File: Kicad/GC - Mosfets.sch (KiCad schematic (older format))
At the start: 15 parts, among them Q1 IRFB7530, Q2 IRFB7530, Q3 IRFB7530, Q4 IRFB7530, Q5 IRFB7530, Q6 IRFB7530

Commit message: Passives changed from 0805 to 0603
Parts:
- Q1, Q2, Q3, Q4, Q5, Q6: footprint TO_SOT_Packages_THT:TO-220-3_Horizontal -> Romain:TO-220-3_Horizontal
- R1, R10, R11, R12, R13, R2, R7, R8, R9: footprint Resistors_SMD:R_0805 -> Resistors_SMD:R_0603
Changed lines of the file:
@@
 F 0 "R13" V 7350 4150 50  0000 C CNN
 F 1 "39k" V 7250 4150 50  0000 C CNN
-F 2 "Resistors_SMD:R_0805" H 7250 4150 60  0001 C CNN
+F 2 "Resistors_SMD:R_0603" H 7250 4150 60  0001 C CNN
 F 3 "" H 7250 4150 60  0001 C CNN
 	1    7250 4150
@@
 F 0 "R7" V 4200 4150 50  0000 C CNN
 F 1 "39k" V 4100 4150 50  0000 C CNN
-F 2 "Resistors_SMD:R_0805" H 4100 4150 60  0001 C CNN
+F 2 "Resistors_SMD:R_0603" H 4100 4150 60  0001 C CNN
 F 3 "" H 4100 4150 60  0001 C CNN
 	1    4100 4150
@@
 F 0 "Q1" H 4210 3070 60  0000 R CNN
 F 1 "IRFB7530" V 4450 3100 60  0000 R CNN
-F 2 "TO_SOT_Packages_THT:TO-220-3_Horizontal" H 4200 2900 60  0001 C CNN
+F 2 "Romain:TO-220-3_Horizontal" H 4200 2900 60  0001 C CNN
 F 3 "IRFB7530" H 4200 2900 60  0001 C CNN
 F 4 "IRFB7530" H 4200 2900 50  0001 C CNN "mfg#"
@@
 F 0 "Q2" H 4210 4020 60  0000 R CNN
 F 1 "IRFB7530" V 4450 4050 60  0000 R CNN
-F 2 "TO_SOT_Packages_THT:TO-220-3_Horizontal" H 4200 3850 60  0001 C CNN
+F 2 "Romain:TO-220-3_Horizontal" H 4200 3850 60  0001 C CNN
 F 3 "IRFB7530" H 4200 3850 60  0001 C CNN
 F 4 "IRFB7530" H 4200 3850 50  0001 C CNN "mfg#"
@@
 F 0 "R2" V 3750 3850 50  0000 C CNN
 F 1 "4R7" V 3650 3850 50  0000 C CNN
-F 2 "Resistors_SMD:R_0805" H 3650 3850 60  0001 C CNN
+F 2 "Resistors_SMD:R_0603" H 3650 3850 60  0001 C CNN
 F 3 "" H 3650 3850 60  0001 C CNN
 	1    3650 3850
@@
 F 0 "R1" V 3750 2900 50  0000 C CNN
 F 1 "4R7" V 3650 2900 50  0000 C CNN
-F 2 "Resistors_SMD:R_0805" H 3650 2900 60  0001 C CNN
+F 2 "Resistors_SMD:R_0603" H 3650 2900 60  0001 C CNN
 F 3 "" H 3650 2900 60  0001 C CNN
 	1    3650 2900
@@
 F 0 "R8" V 5300 2900 50  0000 C CNN
 F 1 "4R7" V 5200 2900 50  0000 C CNN
-F 2 "Resistors_SMD:R_0805" H 5200 2900 60  0001 C CNN
+F 2 "Resistors_SMD:R_0603" H 5200 2900 60  0001 C CNN
 F 3 "" H 5200 2900 60  0001 C CNN
 	1    5200 2900
@@
 F 0 "R9" V 5300 3850 50  0000 C CNN
 F 1 "4R7" V 5200 3850 50  0000 C CNN
-F 2 "Resistors_SMD:R_0805" H 5200 3850 60  0001 C CNN
+F 2 "Resistors_SMD:R_0603" H 5200 3850 60  0001 C CNN
 F 3 "" H 5200 3850 60  0001 C CNN
 	1    5200 3850
@@
 F 0 "Q4" H 5760 4020 60  0000 R CNN
 F 1 "IRFB7530" V 6000 4050 60  0000 R CNN
-F 2 "TO_SOT_Packages_THT:TO-220-3_Horizontal" H 5750 3850 60  0001 C CNN
+F 2 "Romain:TO-220-3_Horizontal" H 5750 3850 60  0001 C CNN
 F 3 "IRFB7530" H 5750 3850 60  0001 C CNN
 F 4 "IRFB7530" H 5750 3850 50  0001 C CNN "mfg#"
@@
 F 0 "Q3" H 5760 3070 60  0000 R CNN
 F 1 "IRFB7530" V 6000 3100 60  0000 R CNN
-F 2 "TO_SOT_Packages_THT:TO-220-3_Horizontal" H 5750 2900 60  0001 C CNN
+F 2 "Romain:TO-220-3_Horizontal" H 5750 2900 60  0001 C CNN
 F 3 "IRFB7530" H 5750 2900 60  0001 C CNN
 F 4 "IRFB7530" H 5750 2900 50  0001 C CNN "mfg#"
@@
 F 0 "Q5" H 7360 3070 60  0000 R CNN
 F 1 "IRFB7530" V 7600 3100 60  0000 R CNN
-F 2 "TO_SOT_Packages_THT:TO-220-3_Horizontal" H 7350 2900 60  0001 C CNN
+F 2 "Romain:TO-220-3_Horizontal" H 7350 2900 60  0001 C CNN
 F 3 "IRFB7530" H 7350 2900 60  0001 C CNN
 F 4 "IRFB7530" H 7350 2900 50  0001 C CNN "mfg#"
@@
 F 0 "Q6" H 7360 4020 60  0000 R CNN
 F 1 "IRFB7530" V 7600 4050 60  0000 R CNN
-F 2 "TO_SOT_Packages_THT:TO-220-3_Horizontal" H 7350 3850 60  0001 C CNN
+F 2 "Romain:TO-220-3_Horizontal" H 7350 3850 60  0001 C CNN
 F 3 "IRFB7530" H 7350 3850 60  0001 C CNN
 F 4 "IRFB7530" H 7350 3850 50  0001 C CNN "mfg#"
@@
 F 0 "R12" V 6900 3850 50  0000 C CNN
 F 1 "4R7" V 6800 3850 50  0000 C CNN
-F 2 "Resistors_SMD:R_0805" H 6800 3850 60  0001 C CNN
+F 2 "Resistors_SMD:R_0603" H 6800 3850 60  0001 C CNN
 F 3 "" H 6800 3850 60  0001 C CNN
 	1    6800 3850
@@
 F 0 "R11" V 6900 2900 50  0000 C CNN
 F 1 "4R7" V 6800 2900 50  0000 C CNN
-F 2 "Resistors_SMD:R_0805" H 6800 2900 60  0001 C CNN
+F 2 "Resistors_SMD:R_0603" H 6800 2900 60  0001 C CNN
 F 3 "" H 6800 2900 60  0001 C CNN
 	1    6800 2900
@@
 F 0 "R10" V 5100 4150 50  0000 C CNN
 F 1 "39k" V 5200 4150 50  0000 C CNN
-F 2 "Resistors_SMD:R_0805" H 5200 4150 60  0001 C CNN
+F 2 "Resistors_SMD:R_0603" H 5200 4150 60  0001 C CNN
 F 3 "" H 5200 4150 60  0001 C CNN
 	1    5200 4150

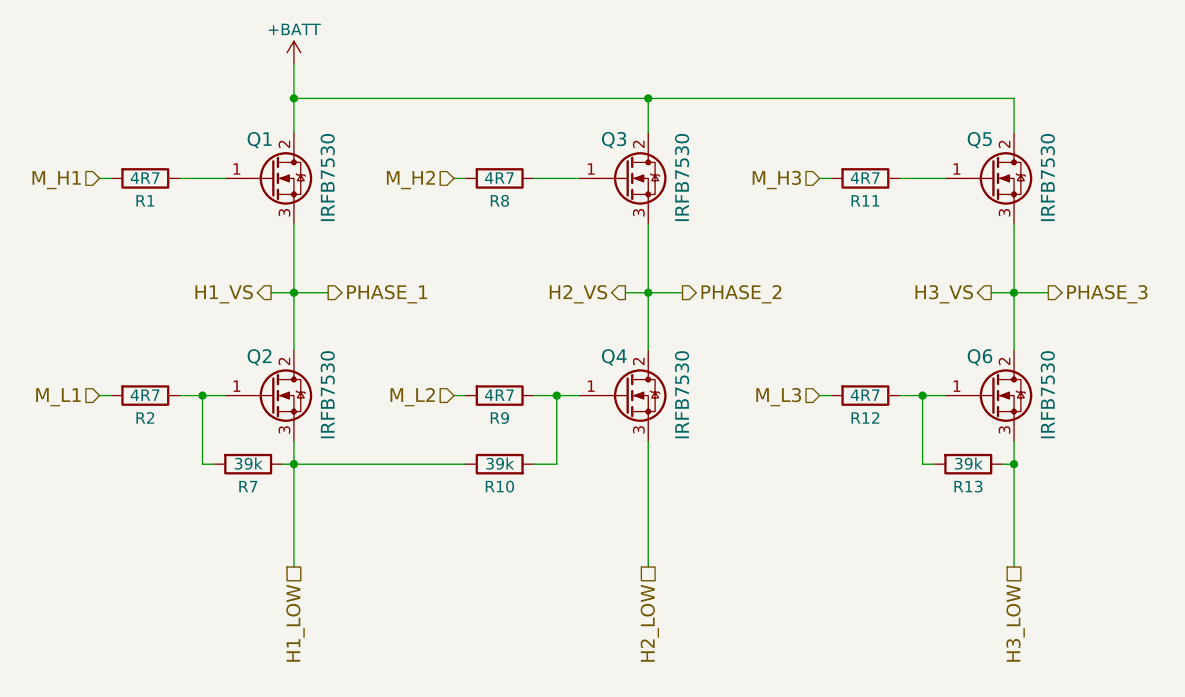
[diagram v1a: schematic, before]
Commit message: Components placed
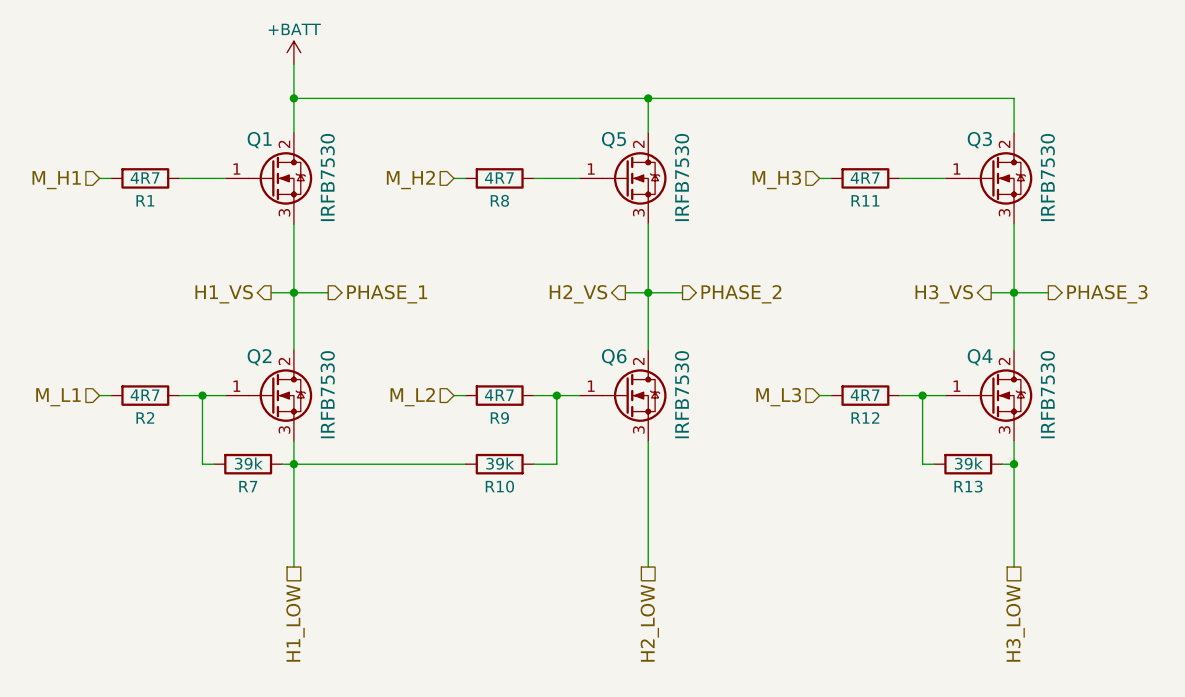
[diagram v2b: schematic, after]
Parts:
- renumbered Q5 to Q3, Q6 to Q4, Q3 to Q5, Q4 to Q6
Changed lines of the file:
@@
 $EndComp
 $Comp
-L Device:Q_NMOS_GDS Q4
+L Device:Q_NMOS_GDS Q6
 U 1 1 53F8E66C
 P 5750 3850
-F 0 "Q4" H 5760 4020 60  0000 R CNN
+F 0 "Q6" H 5760 4020 60  0000 R CNN
 F 1 "IRFB7530" V 6000 4050 60  0000 R CNN
 F 2 "Romain:TO-220-3_Horizontal" H 5750 3850 60  0001 C CNN
@@
 $EndComp
 $Comp
-L Device:Q_NMOS_GDS Q3
+L Device:Q_NMOS_GDS Q5
 U 1 1 53F8E673
 P 5750 2900
-F 0 "Q3" H 5760 3070 60  0000 R CNN
+F 0 "Q5" H 5760 3070 60  0000 R CNN
 F 1 "IRFB7530" V 6000 3100 60  0000 R CNN
 F 2 "Romain:TO-220-3_Horizontal" H 5750 2900 60  0001 C CNN
@@
 $EndComp
 $Comp
-L Device:Q_NMOS_GDS Q5
+L Device:Q_NMOS_GDS Q3
 U 1 1 53F8E67A
 P 7350 2900
-F 0 "Q5" H 7360 3070 60  0000 R CNN
+F 0 "Q3" H 7360 3070 60  0000 R CNN
 F 1 "IRFB7530" V 7600 3100 60  0000 R CNN
 F 2 "Romain:TO-220-3_Horizontal" H 7350 2900 60  0001 C CNN
@@
 $EndComp
 $Comp
-L Device:Q_NMOS_GDS Q6
+L Device:Q_NMOS_GDS Q4
 U 1 1 53F8E681
 P 7350 3850
-F 0 "Q6" H 7360 4020 60  0000 R CNN
+F 0 "Q4" H 7360 4020 60  0000 R CNN
 F 1 "IRFB7530" V 7600 4050 60  0000 R CNN
 F 2 "Romain:TO-220-3_Horizontal" H 7350 3850 60  0001 C CNN

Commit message: Adjusting capacitor size/value
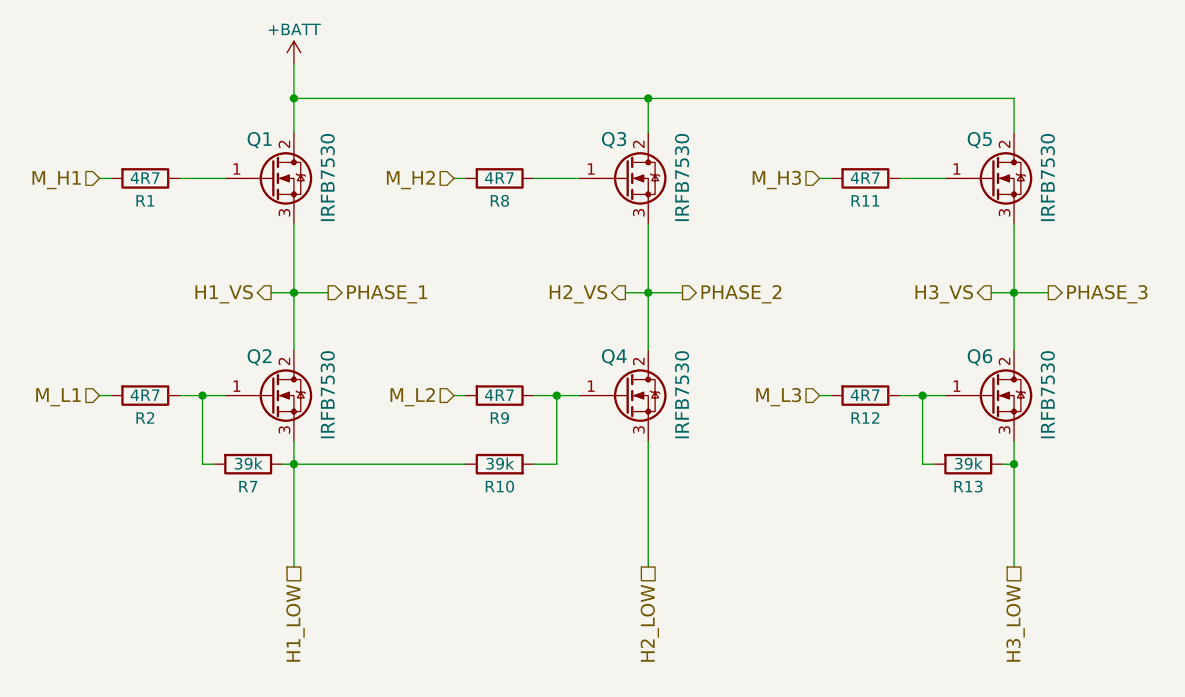
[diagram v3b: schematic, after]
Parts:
- renumbered Q5 to Q3, Q6 to Q4, Q3 to Q5, Q4 to Q6
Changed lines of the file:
@@
 $EndComp
 $Comp
-L Device:Q_NMOS_GDS Q6
+L Device:Q_NMOS_GDS Q4
 U 1 1 53F8E66C
 P 5750 3850
-F 0 "Q6" H 5760 4020 60  0000 R CNN
+F 0 "Q4" H 5760 4020 60  0000 R CNN
 F 1 "IRFB7530" V 6000 4050 60  0000 R CNN
 F 2 "Romain:TO-220-3_Horizontal" H 5750 3850 60  0001 C CNN
@@
 $EndComp
 $Comp
-L Device:Q_NMOS_GDS Q5
+L Device:Q_NMOS_GDS Q3
 U 1 1 53F8E673
 P 5750 2900
-F 0 "Q5" H 5760 3070 60  0000 R CNN
+F 0 "Q3" H 5760 3070 60  0000 R CNN
 F 1 "IRFB7530" V 6000 3100 60  0000 R CNN
 F 2 "Romain:TO-220-3_Horizontal" H 5750 2900 60  0001 C CNN
@@
 $EndComp
 $Comp
-L Device:Q_NMOS_GDS Q3
+L Device:Q_NMOS_GDS Q5
 U 1 1 53F8E67A
 P 7350 2900
-F 0 "Q3" H 7360 3070 60  0000 R CNN
+F 0 "Q5" H 7360 3070 60  0000 R CNN
 F 1 "IRFB7530" V 7600 3100 60  0000 R CNN
 F 2 "Romain:TO-220-3_Horizontal" H 7350 2900 60  0001 C CNN
@@
 $EndComp
 $Comp
-L Device:Q_NMOS_GDS Q4
+L Device:Q_NMOS_GDS Q6
 U 1 1 53F8E681
 P 7350 3850
-F 0 "Q4" H 7360 4020 60  0000 R CNN
+F 0 "Q6" H 7360 4020 60  0000 R CNN
 F 1 "IRFB7530" V 7600 4050 60  0000 R CNN
 F 2 "Romain:TO-220-3_Horizontal" H 7350 3850 60  0001 C CNN

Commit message: Fixed libraries issues
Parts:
- Q1, Q2, Q3, Q4, Q5, Q6: footprint Romain:TO-220-3_Horizontal -> Gouach-Controller:TO-220-3_Horizontal; symbol Device:Q_NMOS_GDS -> Gouach_Controller-rescue:Q_NMOS_GDS-Device
- R1, R10, R11, R12, R13, R2, R7, R8, R9: footprint Resistors_SMD:R_0603 -> Resistor_SMD:R_0603_1608Metric; symbol Device:R -> Gouach_Controller-rescue:R-Device
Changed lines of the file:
@@
 $EndDescr
 $Comp
-L Device:R R13
+L Gouach_Controller-rescue:R-Device R13
 U 1 1 53F8E60B
 P 7250 4150
 F 0 "R13" V 7350 4150 50  0000 C CNN
 F 1 "39k" V 7250 4150 50  0000 C CNN
-F 2 "Resistors_SMD:R_0603" H 7250 4150 60  0001 C CNN
+F 2 "Resistor_SMD:R_0603_1608Metric" H 7250 4150 60  0001 C CNN
 F 3 "" H 7250 4150 60  0001 C CNN
 	1    7250 4150
@@
 $EndComp
 $Comp
-L Device:R R7
+L Gouach_Controller-rescue:R-Device R7
 U 1 1 53F8E612
 P 4100 4150
 F 0 "R7" V 4200 4150 50  0000 C CNN
 F 1 "39k" V 4100 4150 50  0000 C CNN
-F 2 "Resistors_SMD:R_0603" H 4100 4150 60  0001 C CNN
+F 2 "Resistor_SMD:R_0603_1608Metric" H 4100 4150 60  0001 C CNN
 F 3 "" H 4100 4150 60  0001 C CNN
 	1    4100 4150
@@
 $EndComp
 $Comp
-L Device:Q_NMOS_GDS Q1
+L Gouach_Controller-rescue:Q_NMOS_GDS-Device Q1
 U 1 1 53F8E63D
 P 4200 2900
 F 0 "Q1" H 4210 3070 60  0000 R CNN
 F 1 "IRFB7530" V 4450 3100 60  0000 R CNN
-F 2 "Romain:TO-220-3_Horizontal" H 4200 2900 60  0001 C CNN
+F 2 "Gouach-Controller:TO-220-3_Horizontal" H 4200 2900 60  0001 C CNN
 F 3 "IRFB7530" H 4200 2900 60  0001 C CNN
 F 4 "IRFB7530" H 4200 2900 50  0001 C CNN "mfg#"
@@
 $EndComp
 $Comp
-L Device:Q_NMOS_GDS Q2
+L Gouach_Controller-rescue:Q_NMOS_GDS-Device Q2
 U 1 1 53F8E644
 P 4200 3850
 F 0 "Q2" H 4210 4020 60  0000 R CNN
 F 1 "IRFB7530" V 4450 4050 60  0000 R CNN
-F 2 "Romain:TO-220-3_Horizontal" H 4200 3850 60  0001 C CNN
+F 2 "Gouach-Controller:TO-220-3_Horizontal" H 4200 3850 60  0001 C CNN
 F 3 "IRFB7530" H 4200 3850 60  0001 C CNN
 F 4 "IRFB7530" H 4200 3850 50  0001 C CNN "mfg#"
@@
 $EndComp
 $Comp
-L Device:R R2
+L Gouach_Controller-rescue:R-Device R2
 U 1 1 53F8E64B
 P 3650 3850
 F 0 "R2" V 3750 3850 50  0000 C CNN
 F 1 "4R7" V 3650 3850 50  0000 C CNN
-F 2 "Resistors_SMD:R_0603" H 3650 3850 60  0001 C CNN
+F 2 "Resistor_SMD:R_0603_1608Metric" H 3650 3850 60  0001 C CNN
 F 3 "" H 3650 3850 60  0001 C CNN
 	1    3650 3850
@@
 $EndComp
 $Comp
-L Device:R R1
+L Gouach_Controller-rescue:R-Device R1
 U 1 1 53F8E652
 P 3650 2900
 F 0 "R1" V 3750 2900 50  0000 C CNN
 F 1 "4R7" V 3650 2900 50  0000 C CNN
-F 2 "Resistors_SMD:R_0603" H 3650 2900 60  0001 C CNN
+F 2 "Resistor_SMD:R_0603_1608Metric" H 3650 2900 60  0001 C CNN
 F 3 "" H 3650 2900 60  0001 C CNN
 	1    3650 2900
@@
 $EndComp
 $Comp
-L Device:R R8
+L Gouach_Controller-rescue:R-Device R8
 U 1 1 53F8E65E
 P 5200 2900
 F 0 "R8" V 5300 2900 50  0000 C CNN
 F 1 "4R7" V 5200 2900 50  0000 C CNN
-F 2 "Resistors_SMD:R_0603" H 5200 2900 60  0001 C CNN
+F 2 "Resistor_SMD:R_0603_1608Metric" H 5200 2900 60  0001 C CNN
 F 3 "" H 5200 2900 60  0001 C CNN
 	1    5200 2900
@@
 $EndComp
 $Comp
-L Device:R R9
+L Gouach_Controller-rescue:R-Device R9
 U 1 1 53F8E665
 P 5200 3850
 F 0 "R9" V 5300 3850 50  0000 C CNN
 F 1 "4R7" V 5200 3850 50  0000 C CNN
-F 2 "Resistors_SMD:R_0603" H 5200 3850 60  0001 C CNN
+F 2 "Resistor_SMD:R_0603_1608Metric" H 5200 3850 60  0001 C CNN
 F 3 "" H 5200 3850 60  0001 C CNN
 	1    5200 3850
@@
 $EndComp
 $Comp
-L Device:Q_NMOS_GDS Q4
+L Gouach_Controller-rescue:Q_NMOS_GDS-Device Q4
 U 1 1 53F8E66C
 P 5750 3850
 F 0 "Q4" H 5760 4020 60  0000 R CNN
 F 1 "IRFB7530" V 6000 4050 60  0000 R CNN
-F 2 "Romain:TO-220-3_Horizontal" H 5750 3850 60  0001 C CNN
+F 2 "Gouach-Controller:TO-220-3_Horizontal" H 5750 3850 60  0001 C CNN
 F 3 "IRFB7530" H 5750 3850 60  0001 C CNN
 F 4 "IRFB7530" H 5750 3850 50  0001 C CNN "mfg#"
@@
 $EndComp
 $Comp
-L Device:Q_NMOS_GDS Q3
+L Gouach_Controller-rescue:Q_NMOS_GDS-Device Q3
 U 1 1 53F8E673
 P 5750 2900
 F 0 "Q3" H 5760 3070 60  0000 R CNN
 F 1 "IRFB7530" V 6000 3100 60  0000 R CNN
-F 2 "Romain:TO-220-3_Horizontal" H 5750 2900 60  0001 C CNN
+F 2 "Gouach-Controller:TO-220-3_Horizontal" H 5750 2900 60  0001 C CNN
 F 3 "IRFB7530" H 5750 2900 60  0001 C CNN
 F 4 "IRFB7530" H 5750 2900 50  0001 C CNN "mfg#"
@@
 $EndComp
 $Comp
-L Device:Q_NMOS_GDS Q5
+L Gouach_Controller-rescue:Q_NMOS_GDS-Device Q5
 U 1 1 53F8E67A
 P 7350 2900
 F 0 "Q5" H 7360 3070 60  0000 R CNN
 F 1 "IRFB7530" V 7600 3100 60  0000 R CNN
-F 2 "Romain:TO-220-3_Horizontal" H 7350 2900 60  0001 C CNN
+F 2 "Gouach-Controller:TO-220-3_Horizontal" H 7350 2900 60  0001 C CNN
 F 3 "IRFB7530" H 7350 2900 60  0001 C CNN
 F 4 "IRFB7530" H 7350 2900 50  0001 C CNN "mfg#"
@@
 $EndComp
 $Comp
-L Device:Q_NMOS_GDS Q6
+L Gouach_Controller-rescue:Q_NMOS_GDS-Device Q6
 U 1 1 53F8E681
 P 7350 3850
 F 0 "Q6" H 7360 4020 60  0000 R CNN
 F 1 "IRFB7530" V 7600 4050 60  0000 R CNN
-F 2 "Romain:TO-220-3_Horizontal" H 7350 3850 60  0001 C CNN
+F 2 "Gouach-Controller:TO-220-3_Horizontal" H 7350 3850 60  0001 C CNN
 F 3 "IRFB7530" H 7350 3850 60  0001 C CNN
 F 4 "IRFB7530" H 7350 3850 50  0001 C CNN "mfg#"
@@
 $EndComp
 $Comp
-L Device:R R12
+L Gouach_Controller-rescue:R-Device R12
 U 1 1 53F8E688
 P 6800 3850
 F 0 "R12" V 6900 3850 50  0000 C CNN
 F 1 "4R7" V 6800 3850 50  0000 C CNN
-F 2 "Resistors_SMD:R_0603" H 6800 3850 60  0001 C CNN
+F 2 "Resistor_SMD:R_0603_1608Metric" H 6800 3850 60  0001 C CNN
 F 3 "" H 6800 3850 60  0001 C CNN
 	1    6800 3850
@@
 $EndComp
 $Comp
-L Device:R R11
+L Gouach_Controller-rescue:R-Device R11
 U 1 1 53F8E68F
 P 6800 2900
 F 0 "R11" V 6900 2900 50  0000 C CNN
 F 1 "4R7" V 6800 2900 50  0000 C CNN
-F 2 "Resistors_SMD:R_0603" H 6800 2900 60  0001 C CNN
+F 2 "Resistor_SMD:R_0603_1608Metric" H 6800 2900 60  0001 C CNN
 F 3 "" H 6800 2900 60  0001 C CNN
 	1    6800 2900
@@
 $EndComp
 $Comp
-L Device:R R10
+L Gouach_Controller-rescue:R-Device R10
 U 1 1 53F8E69C
 P 5200 4150
 F 0 "R10" V 5100 4150 50  0000 C CNN
 F 1 "39k" V 5200 4150 50  0000 C CNN
-F 2 "Resistors_SMD:R_0603" H 5200 4150 60  0001 C CNN
+F 2 "Resistor_SMD:R_0603_1608Metric" H 5200 4150 60  0001 C CNN
 F 3 "" H 5200 4150 60  0001 C CNN
 	1    5200 4150
@@
 	7050 4150 7100 4150
 $Comp
-L power:+BATT #PWR0126
+L Gouach_Controller-rescue:+BATT-power #PWR0126
 U 1 1 5F21FCD0
 P 4300 2400

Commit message: Add Mouser order number
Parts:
- Q1, Q2, Q3, Q4, Q5, Q6: Mouser (none) -> 942-IRFB7530PBF; mfg# IRFB7530 -> (none)
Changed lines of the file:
@@
 F 1 "IRFB7530" V 4450 3100 60  0000 R CNN
 F 2 "Gouach-Controller:TO-220-3_Horizontal" H 4200 2900 60  0001 C CNN
-F 3 "IRFB7530" H 4200 2900 60  0001 C CNN
-F 4 "IRFB7530" H 4200 2900 50  0001 C CNN "mfg#"
+F 3 "https://www.infineon.com/dgdl/irfs7530pbf.pdf?fileId=5546d462533600a4015364c3d98429c3" H 4200 2900 60  0001 C CNN
+F 4 "" H 4200 2900 50  0001 C CNN "mfg#"
+F 5 "942-IRFB7530PBF " H 4200 2900 50  0001 C CNN "Mouser"
 	1    4200 2900
 	1    0    0    -1
@@
 F 1 "IRFB7530" V 4450 4050 60  0000 R CNN
 F 2 "Gouach-Controller:TO-220-3_Horizontal" H 4200 3850 60  0001 C CNN
-F 3 "IRFB7530" H 4200 3850 60  0001 C CNN
-F 4 "IRFB7530" H 4200 3850 50  0001 C CNN "mfg#"
+F 3 "https://www.infineon.com/dgdl/irfs7530pbf.pdf?fileId=5546d462533600a4015364c3d98429c3" H 4200 3850 60  0001 C CNN
+F 4 "" H 4200 3850 50  0001 C CNN "mfg#"
+F 5 "942-IRFB7530PBF " H 4200 3850 50  0001 C CNN "Mouser"
 	1    4200 3850
 	1    0    0    -1
@@
 F 1 "IRFB7530" V 6000 4050 60  0000 R CNN
 F 2 "Gouach-Controller:TO-220-3_Horizontal" H 5750 3850 60  0001 C CNN
-F 3 "IRFB7530" H 5750 3850 60  0001 C CNN
-F 4 "IRFB7530" H 5750 3850 50  0001 C CNN "mfg#"
+F 3 "https://www.infineon.com/dgdl/irfs7530pbf.pdf?fileId=5546d462533600a4015364c3d98429c3" H 5750 3850 60  0001 C CNN
+F 4 "" H 5750 3850 50  0001 C CNN "mfg#"
+F 5 "942-IRFB7530PBF " H 5750 3850 50  0001 C CNN "Mouser"
 	1    5750 3850
 	1    0    0    -1
@@
 F 1 "IRFB7530" V 6000 3100 60  0000 R CNN
 F 2 "Gouach-Controller:TO-220-3_Horizontal" H 5750 2900 60  0001 C CNN
-F 3 "IRFB7530" H 5750 2900 60  0001 C CNN
-F 4 "IRFB7530" H 5750 2900 50  0001 C CNN "mfg#"
+F 3 "https://www.infineon.com/dgdl/irfs7530pbf.pdf?fileId=5546d462533600a4015364c3d98429c3" H 5750 2900 60  0001 C CNN
+F 4 "" H 5750 2900 50  0001 C CNN "mfg#"
+F 5 "942-IRFB7530PBF " H 5750 2900 50  0001 C CNN "Mouser"
 	1    5750 2900
 	1    0    0    -1
@@
 F 1 "IRFB7530" V 7600 3100 60  0000 R CNN
 F 2 "Gouach-Controller:TO-220-3_Horizontal" H 7350 2900 60  0001 C CNN
-F 3 "IRFB7530" H 7350 2900 60  0001 C CNN
-F 4 "IRFB7530" H 7350 2900 50  0001 C CNN "mfg#"
+F 3 "https://www.infineon.com/dgdl/irfs7530pbf.pdf?fileId=5546d462533600a4015364c3d98429c3" H 7350 2900 60  0001 C CNN
+F 4 "" H 7350 2900 50  0001 C CNN "mfg#"
+F 5 "942-IRFB7530PBF " H 7350 2900 50  0001 C CNN "Mouser"
 	1    7350 2900
 	1    0    0    -1
@@
 F 1 "IRFB7530" V 7600 4050 60  0000 R CNN
 F 2 "Gouach-Controller:TO-220-3_Horizontal" H 7350 3850 60  0001 C CNN
-F 3 "IRFB7530" H 7350 3850 60  0001 C CNN
-F 4 "IRFB7530" H 7350 3850 50  0001 C CNN "mfg#"
+F 3 "https://www.infineon.com/dgdl/irfs7530pbf.pdf?fileId=5546d462533600a4015364c3d98429c3" H 7350 3850 60  0001 C CNN
+F 4 "" H 7350 3850 50  0001 C CNN "mfg#"
+F 5 "942-IRFB7530PBF " H 7350 3850 50  0001 C CNN "Mouser"
 	1    7350 3850
 	1    0    0    -1
